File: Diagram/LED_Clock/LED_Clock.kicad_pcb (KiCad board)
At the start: 2 copper layers, 190.5 x 159.4 mm, 79 parts, among them SW1 SW_Push_Dual, U1 ATmega328P-PU, U2 DS3231MZ, U3 MCP23017-E_SP, U4 MCP23017-E_SP, U5 Barreljack, U6 JST4pin, Y1 Crystal

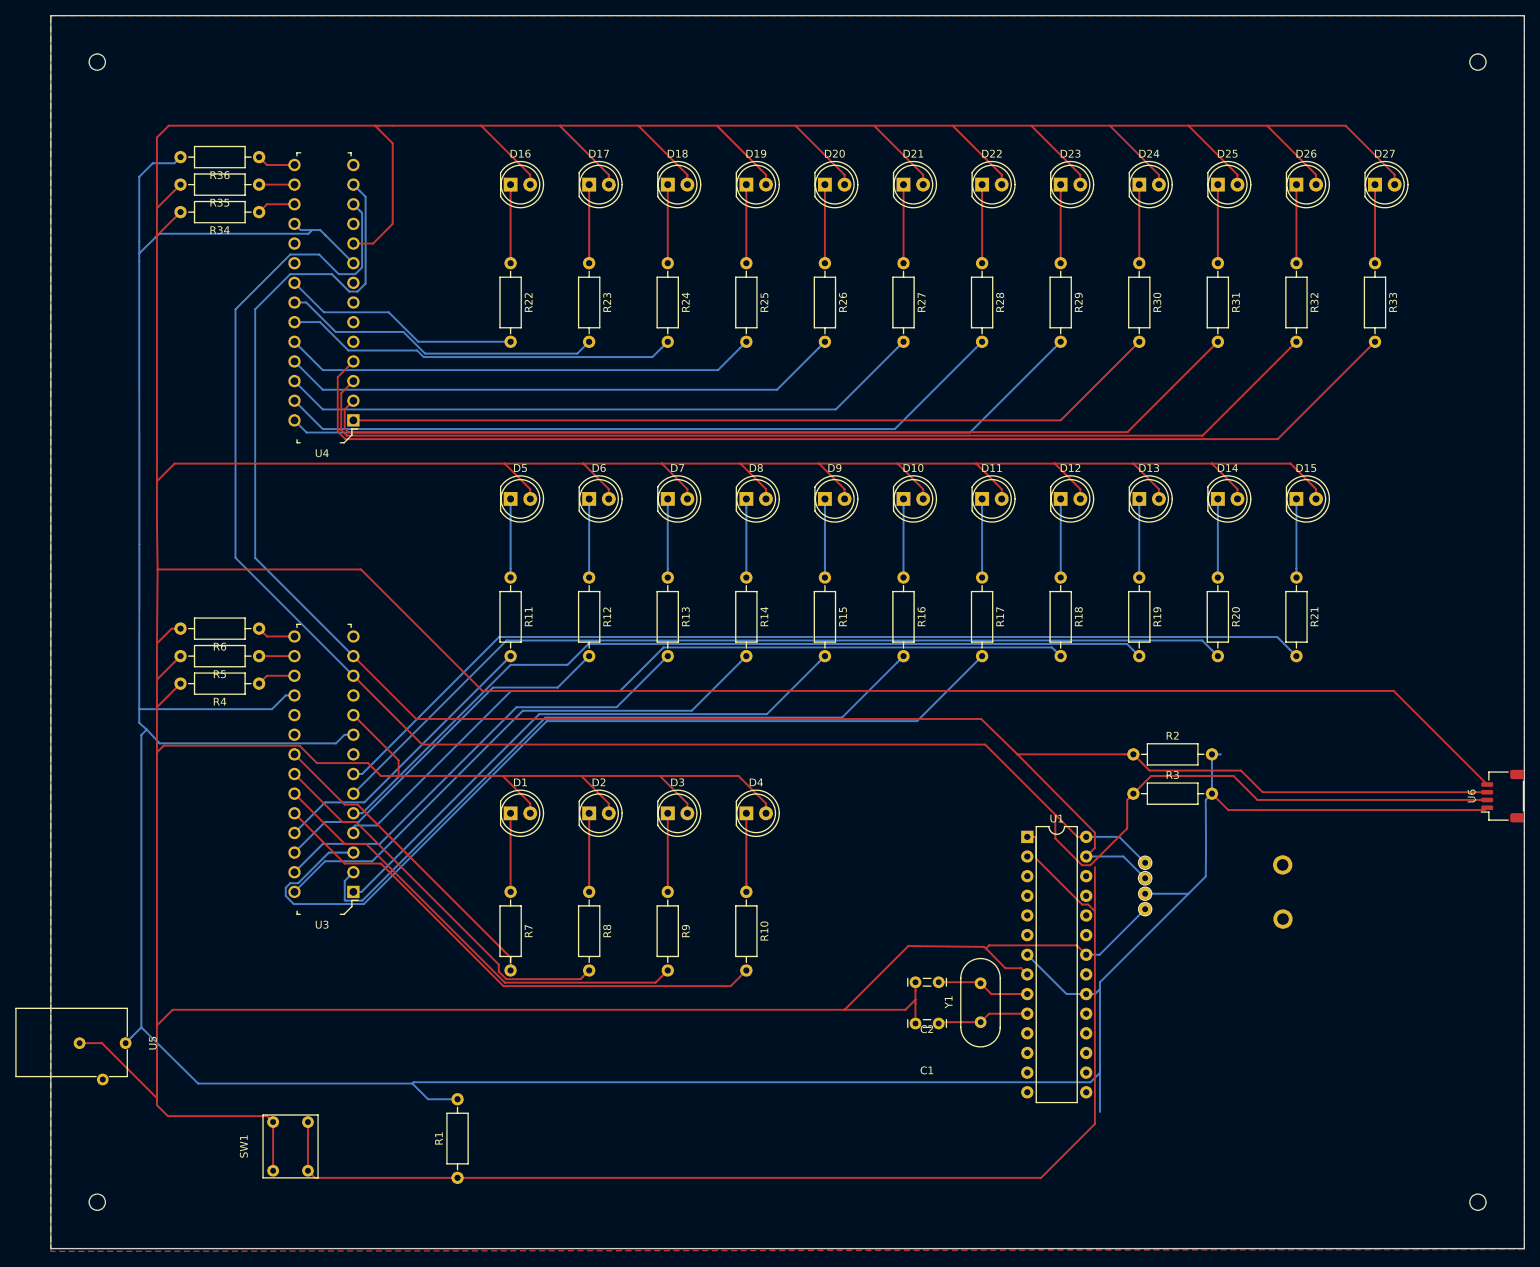
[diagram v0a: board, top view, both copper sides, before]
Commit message: updated
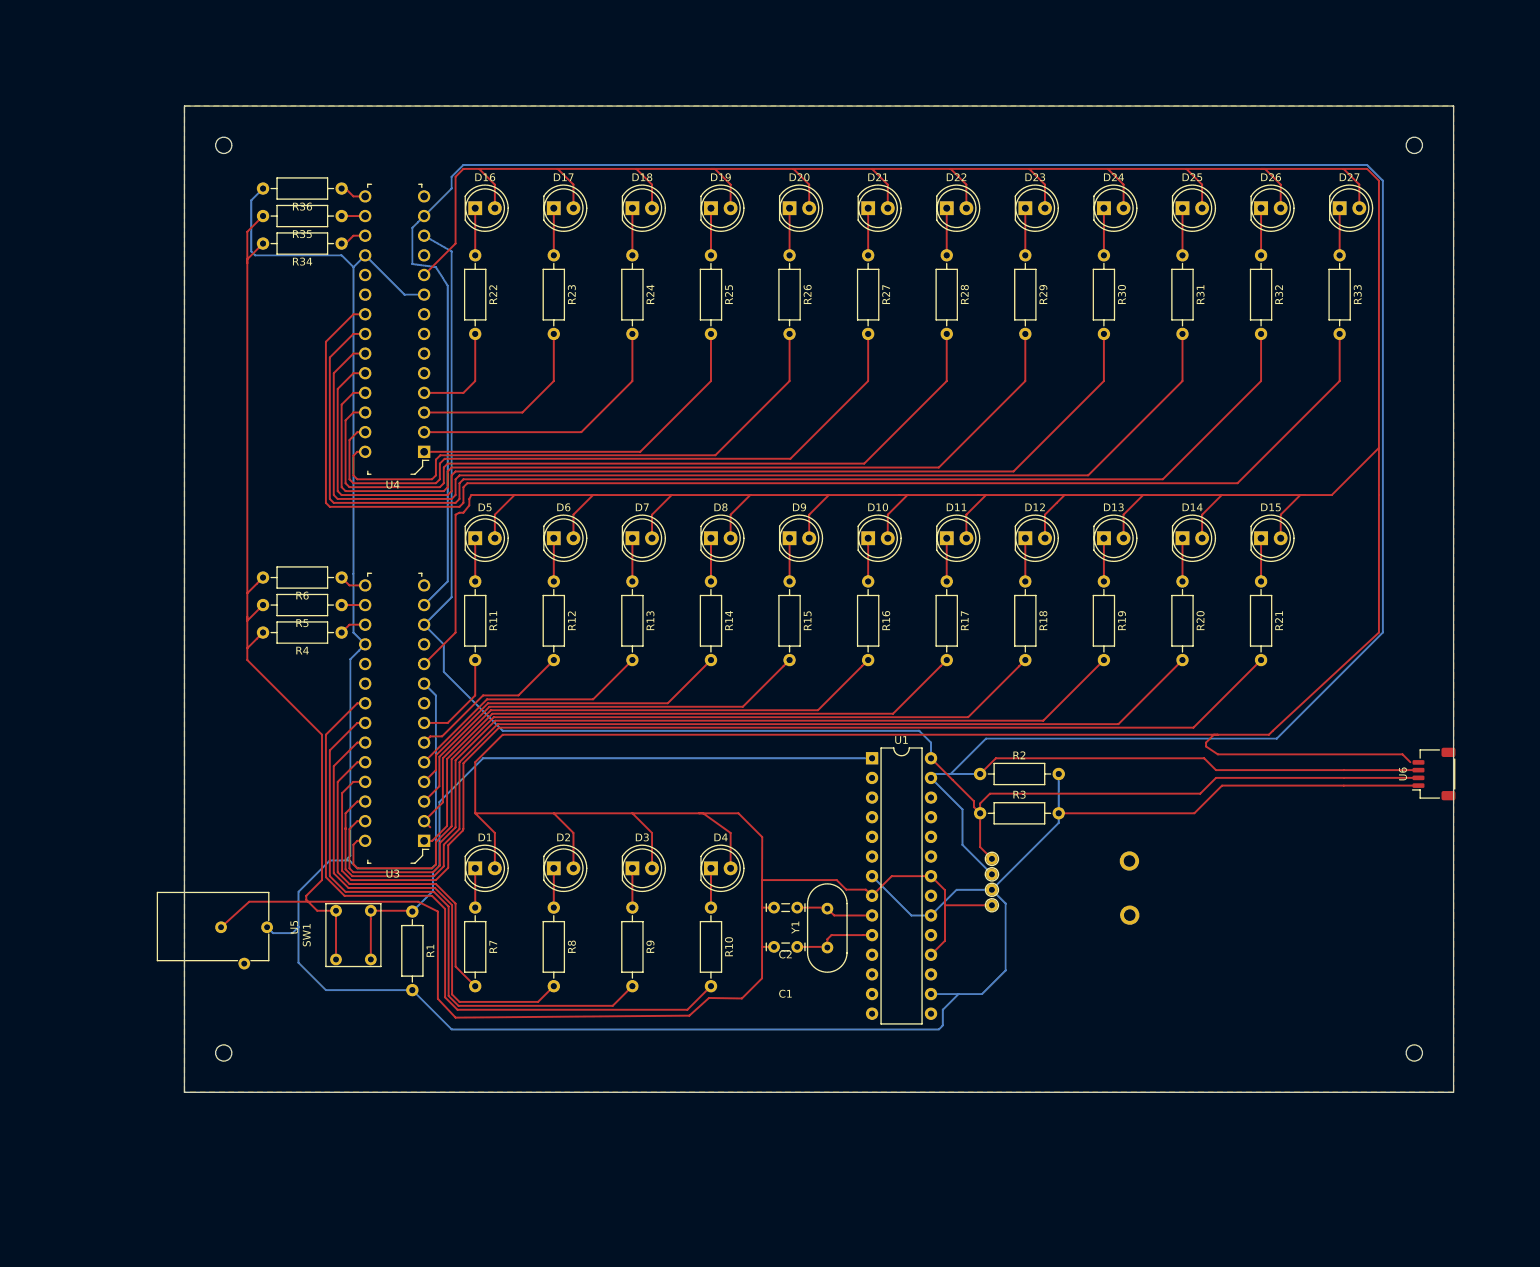
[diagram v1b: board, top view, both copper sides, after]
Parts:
- moved R1 34.9 mm to (84.8, 128.5), turned to 270 degrees
- moved SW1 28.5 mm to (77.2, 131.6)
- moved REF** 25.3 mm to (60.5, 146.8)
- moved U5 23.6 mm to (58.9, 130.6)
- moved U1 22.5 mm to (144.3, 108.7)
- moved Y1 22.0 mm to (138.2, 130.6)
- moved REF** 21.0 mm to (214.4, 146.8)
- moved C1 20.8 mm to (133.1, 133.1)
- moved C2 20.7 mm to (133.1, 128.0)
- moved R2 20.0 mm to (158.2, 110.7)
- moved R3 20.0 mm to (158.2, 115.8)
- moved REF** 19.8 mm to (177.6, 129.0)
- moved REF** 19.8 mm to (177.5, 122.0)
- moved U2 19.8 mm to (159.8, 124.7)
- moved REF** 19.6 mm to (60.5, 29.5)
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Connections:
- net GPB1 renamed Net-(R16-Pad2)
- R15 pad 2: GPB0 -> Net-(R15-Pad2)
- R17 pad 2: GPB2 -> Net-(R17-Pad2)
- R18 pad 2: GPB3 -> Net-(R18-Pad2)
- R19 pad 2: GPB4 -> Net-(R19-Pad2)
- R20 pad 2: GPB5 -> Net-(R20-Pad2)
- R21 pad 2: GPB6 -> Net-(R21-Pad2)
- R30 pad 2: HGPB0 -> Net-(R30-Pad2)
- R31 pad 2: HGPB1 -> Net-(R31-Pad2)
- R32 pad 2: HGPB2 -> Net-(R32-Pad2)
- R33 pad 2: HGPB3 -> Net-(R33-Pad2)
- U1 pad 16: Net-(U1-Pad16) -> +5V
- U1 pad 18: Net-(U1-Pad18) -> GND
- U3 pad 1: GPB0 -> Net-(R17-Pad2)
- U3 pad 21: Net-(R7-Pad2) -> Net-(R10-Pad2)
- U3 pad 22: Net-(R8-Pad2) -> Net-(R9-Pad2)
- U3 pad 23: Net-(R9-Pad2) -> Net-(R8-Pad2)
- U3 pad 24: Net-(R10-Pad2) -> Net-(R7-Pad2)
- U3 pad 25: Net-(R11-Pad2) -> Net-(R21-Pad2)
- U3 pad 26: Net-(R12-Pad2) -> Net-(R20-Pad2)
- U3 pad 27: Net-(R13-Pad2) -> Net-(R19-Pad2)
- U3 pad 28: Net-(R14-Pad2) -> Net-(R18-Pad2)
- U3 pad 3: GPB2 -> Net-(R15-Pad2)
- U3 pad 4: GPB3 -> Net-(R14-Pad2)
- U3 pad 5: GPB4 -> Net-(R13-Pad2)
- U3 pad 6: GPB5 -> Net-(R12-Pad2)
- U3 pad 7: GPB6 -> Net-(R11-Pad2)
- U4 pad 1: HGPB0 -> Net-(R25-Pad2)
- U4 pad 2: HGPB1 -> Net-(R24-Pad2)
- U4 pad 21: Net-(R22-Pad2) -> Net-(R33-Pad2)
- U4 pad 22: Net-(R23-Pad2) -> Net-(R32-Pad2)
- U4 pad 23: Net-(R24-Pad2) -> Net-(R31-Pad2)
- U4 pad 24: Net-(R25-Pad2) -> Net-(R30-Pad2)
- U4 pad 25: Net-(R26-Pad2) -> Net-(R29-Pad2)
- U4 pad 26: Net-(R27-Pad2) -> Net-(R28-Pad2)
- U4 pad 27: Net-(R28-Pad2) -> Net-(R27-Pad2)
- U4 pad 28: Net-(R29-Pad2) -> Net-(R26-Pad2)
- U4 pad 3: HGPB2 -> Net-(R23-Pad2)
- U4 pad 4: HGPB3 -> Net-(R22-Pad2)
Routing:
- net Net-(R33-Pad2): track 0.00 -> 172.7 mm
- net GND: track 1150.4 -> 982.4 mm
- net Net-(R32-Pad2): track 0.00 -> 158.5 mm
- net Net-(R21-Pad2): track 0.00 -> 151.5 mm
- net HGPB3: track 149.6 -> 0.00 mm
- net Net-(R31-Pad2): track 0.00 -> 144.4 mm
- net Net-(R20-Pad2): track 0.00 -> 137.4 mm
- net HGPB2: track 135.8 -> 0.00 mm
- net GPB6: track 130.3 -> 0.00 mm
- net Net-(R30-Pad2): track 0.00 -> 130.3 mm
- net /clock minute/SDA: track 261.5 -> 386.0 mm
- net Net-(R19-Pad2): track 0.00 -> 123.4 mm
- net HGPB1: track 122.0 -> 0.00 mm
- net GPB5: track 120.8 -> 0.00 mm
- net GPB2: track 115.4 -> 0.00 mm
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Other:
- board size 190.5 x 159.4 mm -> 164.1 x 127.5 mm
- rule pad_to_mask_clearance: 0.051 -> 0.00129
- rule solder_mask_min_width: 0.25 -> 0.002565
- rule trace_min: 0.2 -> 0.000152
- rule via_min_drill: 0.3 -> 0.000254
- rule via_min_size: 0.4 -> 0.000508
